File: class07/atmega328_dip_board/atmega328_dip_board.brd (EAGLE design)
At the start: 64.8 x 15.2 mm, 9 parts, among them U1 328P

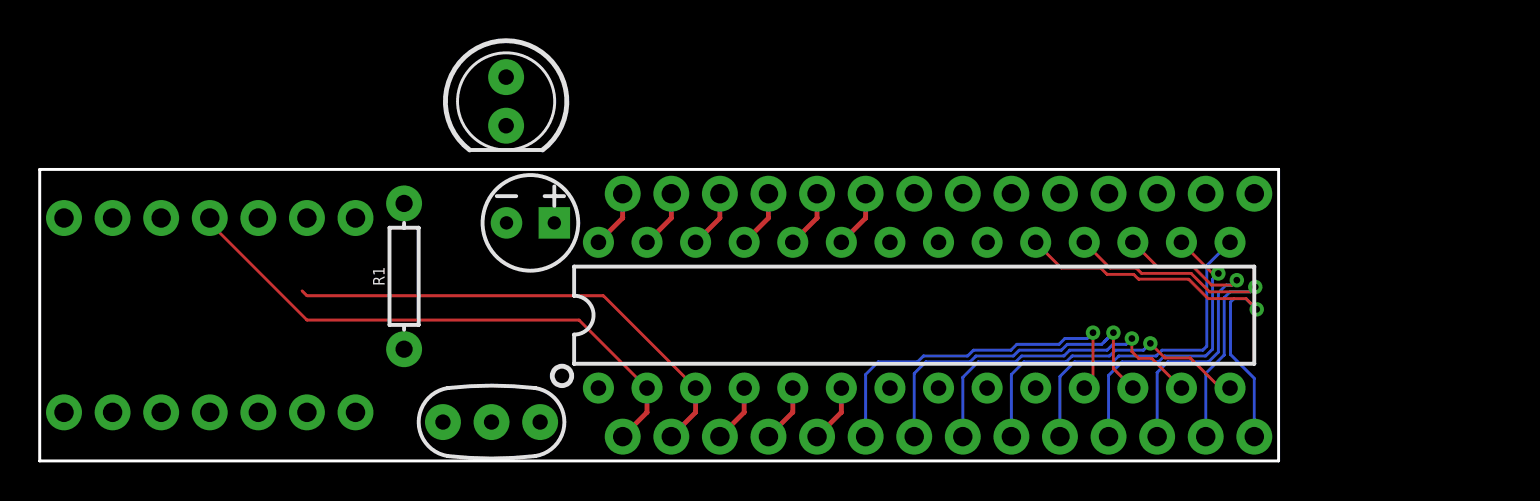
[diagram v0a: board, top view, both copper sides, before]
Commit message: update board
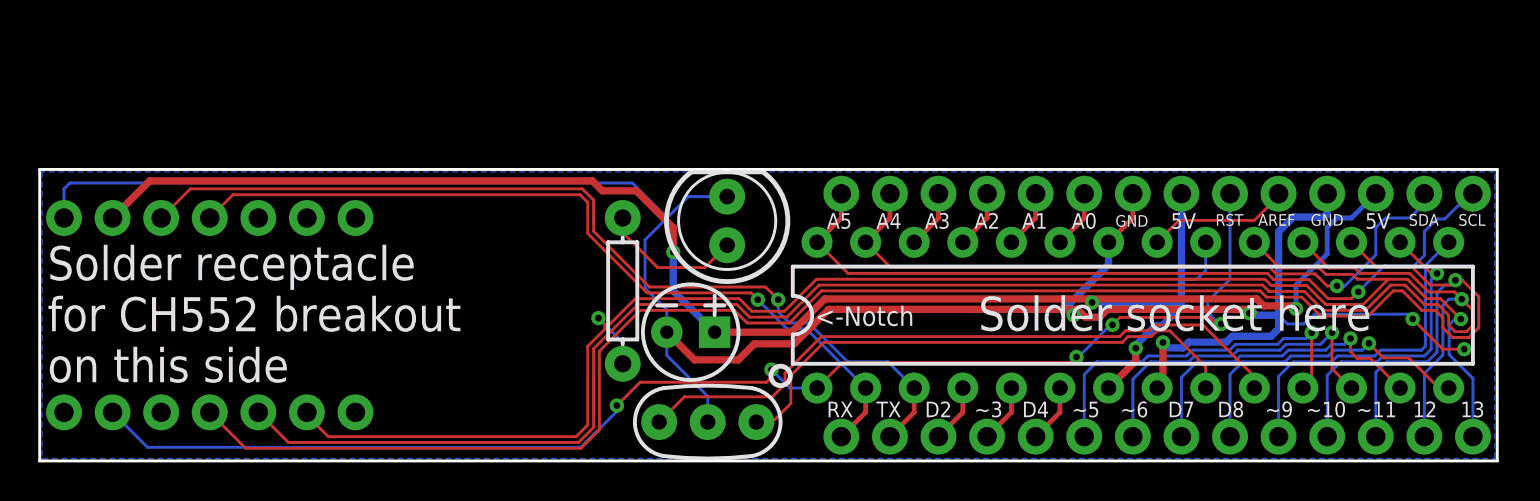
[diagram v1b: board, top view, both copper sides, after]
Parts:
- moved D1 13.1 mm to (35.9, 12.5), turned to 90 degrees
- moved R1 11.5 mm to (30.5, 8.89)
- moved U1 11.4 mm to (57.1, 7.62)
- moved J3 11.4 mm to (41.9, 1.27)
- moved J4 11.4 mm to (41.9, 14.0)
- moved Y1 11.3 mm to (34.9, 2.03), turned to 180 degrees
- moved C1 10.1 mm to (34.0, 6.73)
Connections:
- removed net N$21: J4.7
- removed net N$22: J4.8
- removed net N$23: J4.9
- removed net N$24: J4.10
- removed net N$25: J4.11
- removed net N$26: J4.12
- removed net N$27: J4.13
- removed net N$28: J4.14
- new net N$2: D1.A, R1.P$2
- net 5V: now also C1.1, J4.12, J4.8
- net A4: now also J4.13
- net A5: now also J4.14
- net AREF: now also J4.10
- net D13: now also R1.P$1
- net GND: now also C1.2, D1.K, J4.11, J4.7, Y1.2
- net RESET: now also J4.9
- net XTAL1: now also Y1.1
- net XTAL2: now also Y1.3
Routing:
- net GND: track 0.00 -> 121.7 mm, vias 0 -> 5
- net 5V: track 0.00 -> 96.8 mm, vias 0 -> 4
- net D11: track 17.8 -> 97.1 mm
- net D12: track 19.6 -> 92.6 mm
- net RESET: track 0.00 -> 70.5 mm, vias 0 -> 5
- net D13: track 22.2 -> 87.8 mm, vias 1 -> 2
- net A5: track 3.07 -> 41.6 mm, vias 0 -> 1
- net XTAL2: track 0.00 -> 35.3 mm
- net A4: track 3.07 -> 36.4 mm, vias 0 -> 1
- net XTAL1: track 0.00 -> 28.2 mm
- net D1: track 25.7 -> 48.7 mm, vias 0 -> 1
- net D0: track 29.8 -> 43.0 mm, vias 0 -> 1
- net AREF: track 0.00 -> 7.48 mm
- net N$2: track 0.00 -> 7.46 mm
- net D6: track 18.6 -> 17.7 mm
- added copper zone on layer 16, net GND
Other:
- board size 64.8 x 15.2 mm -> 76.2 x 15.2 mm
- board text added: "12"
- board text added: "13"
- board text added: "5V"
- board text added: "<-Notch"
- board text added: "A0"
- board text added: "A1"
- board text added: "A2"
- board text added: "A3"
- board text added: "A4"
- board text added: "A5"
- board text added: "AREF"
- board text added: "ATmega328 THT Board Arduino Uno Compatible debugWire Debuggable"
- board text added: "D2"
- board text added: "D4"
- board text added: "D7"
- board text added: "D8"
- board text added: "GND"
- board text added: "Prototyping Electronic Devices Deqing 2024"
- board text added: "RST"
- board text added: "RX"
- board text added: "SCL"
- board text added: "SDA"
- board text added: "Solder receptacle for CH552 breakout on this side"
- board text added: "Solder socket here"
- board text added: "TX"
- board text added: "~10"
- board text added: "~11"
- board text added: "~3"
- board text added: "~5"
- board text added: "~6"
- board text added: "~9"
